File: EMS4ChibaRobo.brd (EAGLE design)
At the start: 51 x 51.5 mm, 31 parts, among them CON1 XT60PB-F, CON2 XT60PB-M, CON3 XT60PB-M, Q2 BUZ11BH, U1 V23134J1052D642, U10 MC34063AD, U4 TLP184, U9 XC6206

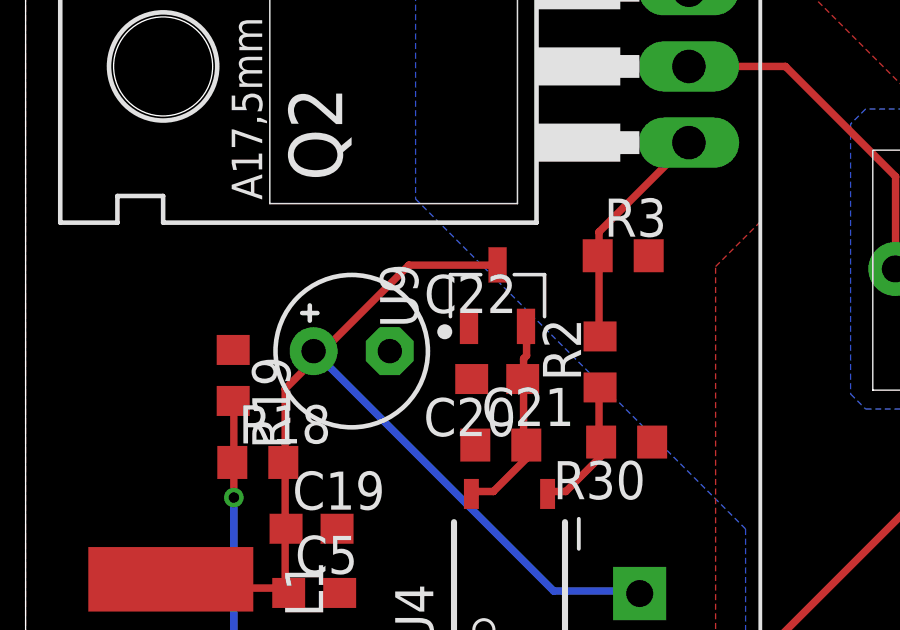
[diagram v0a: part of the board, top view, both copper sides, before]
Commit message: 微調整
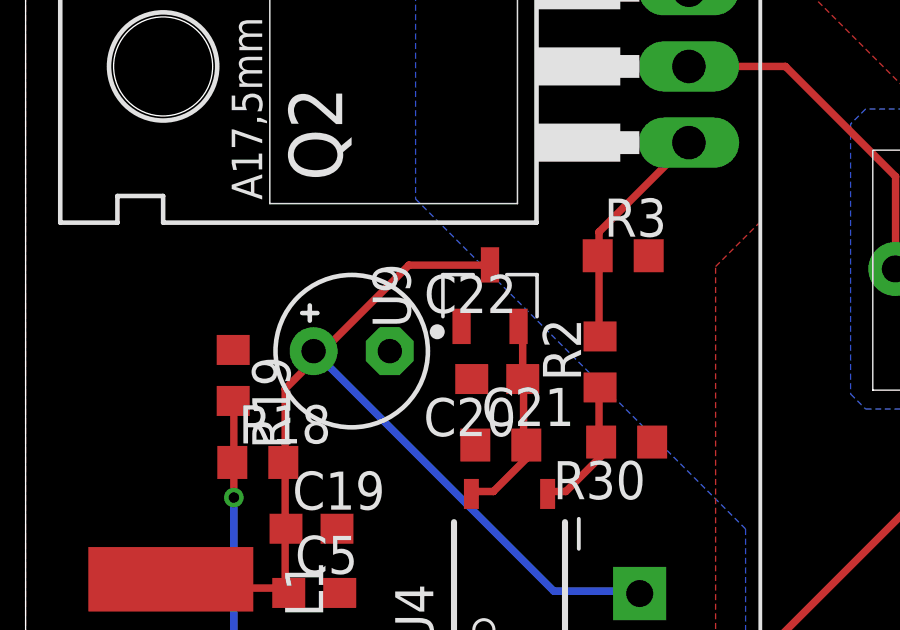
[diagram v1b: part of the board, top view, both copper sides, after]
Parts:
- moved U9 0.25 mm to (15.5, 57.0)
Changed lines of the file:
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@@
 <attribute name="VALUE" x="19.94" y="45.275" size="1.27" layer="27" rot="R90"/>
 </element>
-<element name="U9" library="torex" package="SOT95P240X110-3" package3d_urn="urn:adsk.eagle:package:6993131/1" value="XC6206" x="15.73" y="57.03" smashed="yes" rot="R90">
-<attribute name="NAME" x="13.0864" y="57.03" size="1.27" layer="25" rot="R90" align="bottom-center"/>
-<attribute name="VALUE" x="17.9336" y="57.03" size="1.27" layer="27" rot="R90" align="top-center"/>
+<element name="U9" library="torex" package="SOT95P240X110-3" package3d_urn="urn:adsk.eagle:package:6993131/1" value="XC6206" x="15.48" y="57.03" smashed="yes" rot="R90">
+<attribute name="NAME" x="12.8364" y="57.03" size="1.27" layer="25" rot="R90" align="bottom-center"/>
+<attribute name="VALUE" x="17.6836" y="57.03" size="1.27" layer="27" rot="R90" align="top-center"/>
 </element>
 <element name="C19" library="rcl" library_urn="urn:adsk.eagle:library:334" package="C0603" package3d_urn="urn:adsk.eagle:package:23616/2" value="1u" x="9.53" y="49.26" smashed="yes">
@@
 <contactref element="U9" pad="2"/>
 <contactref element="C20" pad="1"/>
-<wire x1="16.599" y1="54.9276" x2="16.599" y2="54.324" width="0.25" layer="1"/>
-<wire x1="16.6996" y1="55.0282" x2="16.599" y2="54.9276" width="0.25" layer="1"/>
-<wire x1="16.6996" y1="55.9336" x2="16.6996" y2="55.0282" width="0.25" layer="1"/>
-<wire x1="16.599" y1="54.324" x2="16.57" y2="54.25" width="0.25" layer="1"/>
-<wire x1="16.6996" y1="55.9336" x2="16.68" y2="56.0055" width="0.25" layer="1"/>
 <wire x1="15.593" y1="50.5012" x2="14.8888" y2="50.5012" width="0.25" layer="1"/>
 <wire x1="16.6996" y1="51.6078" x2="15.593" y2="50.5012" width="0.25" layer="1"/>
@@
 <wire x1="16.599" y1="54.2234" x2="16.57" y2="54.25" width="0.25" layer="1"/>
 <wire x1="16.599" y1="52.1108" x2="16.69" y2="52.05" width="0.25" layer="1"/>
+<wire x1="16.57" y1="54.25" x2="16.57" y2="55.8655" width="0.25" layer="1"/>
+<wire x1="16.57" y1="55.8655" x2="16.43" y2="56.0055" width="0.25" layer="1"/>
 </signal>
 <signal name="N$30">
@@
 <wire x1="8.551" y1="47.282" x2="8.77" y2="47.12" width="0.25" layer="1"/>
 <wire x1="4.9294" y1="47.4832" x2="4.84" y2="47.575" width="0.25" layer="1"/>
-<wire x1="12.7762" y1="58.0462" x2="15.6936" y2="58.0462" width="0.25" layer="1"/>
+<wire x1="12.7762" y1="58.0462" x2="15.4436" y2="58.0462" width="0.25" layer="1"/>
 <wire x1="9.9594" y1="55.2294" x2="12.7762" y2="58.0462" width="0.25" layer="1"/>
 <wire x1="9.6576" y1="55.2294" x2="9.9594" y2="55.2294" width="0.25" layer="1"/>
-<wire x1="15.6936" y1="58.0462" x2="15.73" y2="58.0545" width="0.25" layer="1"/>
+<wire x1="15.4436" y1="58.0462" x2="15.48" y2="58.0545" width="0.25" layer="1"/>
 <wire x1="9.6576" y1="55.2294" x2="9.6" y2="55.18" width="0.25" layer="1"/>
 <wire x1="17.605" y1="47.1814" x2="20.4218" y2="47.1814" width="0.25" layer="16"/>

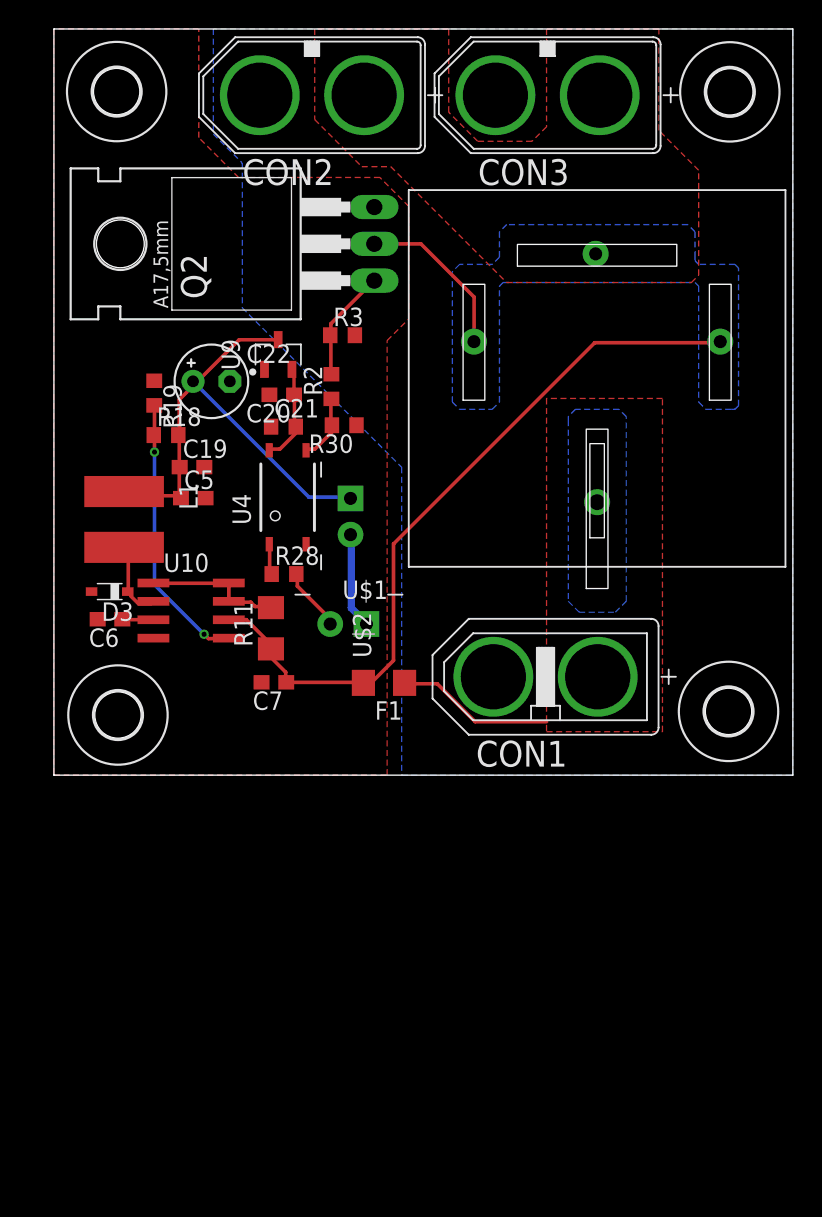
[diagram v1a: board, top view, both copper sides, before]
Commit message: 大幅な設計変更
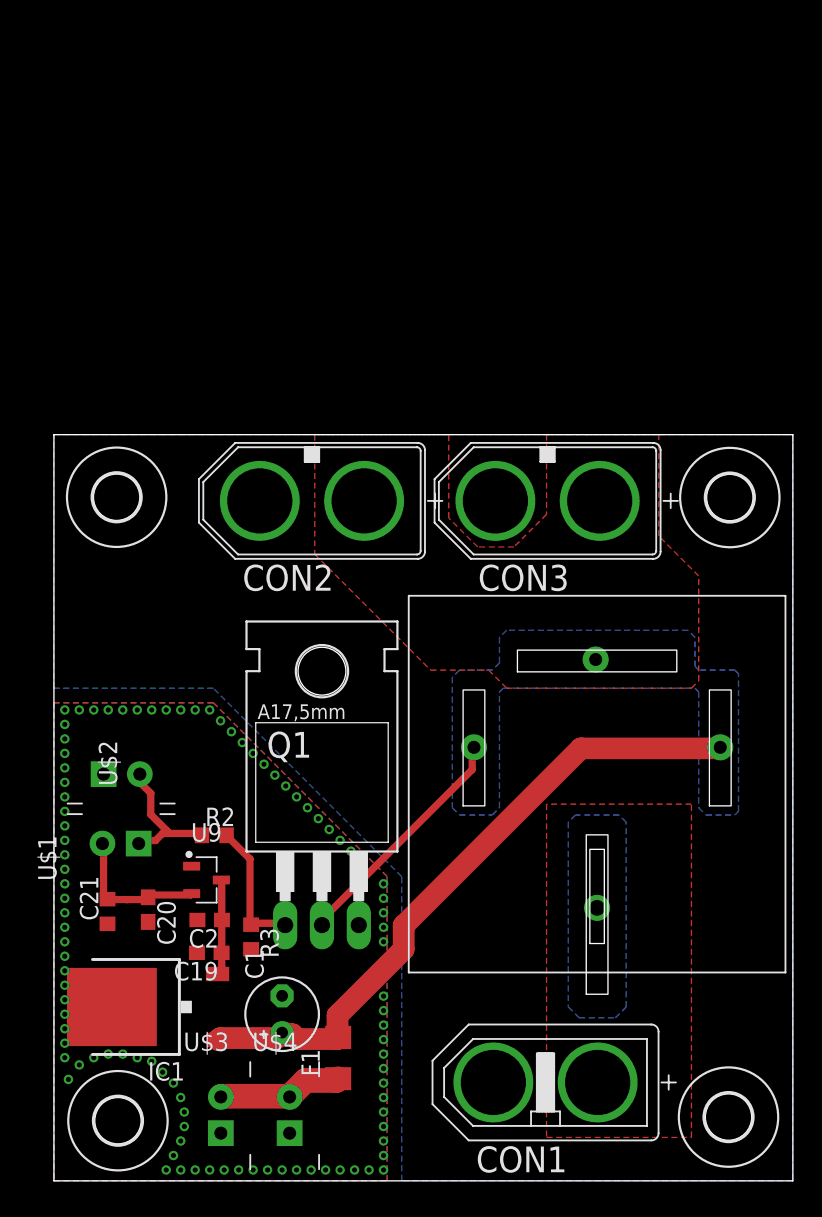
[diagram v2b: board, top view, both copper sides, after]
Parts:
- removed C22: 47u, rcl:E2,5-5
- removed C5, C7: 100n, rcl:C0603
- removed C6: 100p, rcl:C0603
- removed D3: PMEG6010CEJ,115, nexperia:SOD323_ST
- removed L1: L5852, inductors:L5852
- removed Q2: BUZ11BH, transistor-power:TO220BH
- removed R11: 0.68, rcl:R1206
- removed R18: 3.6k, rcl:R0603
- removed R19: 1.2k, rcl:R0603
- removed R28, R30: 1k, rcl:R0603
- removed U10: MC34063AD, mc34063:SOIC8
- removed U4: TLP184, md201x:11-4M1S
- added C1: 22u, rcl:E2,5-5
- added C2: 100n, rcl:C0603
- added IC1: 7805DT, linear:TO252
- added Q1: BUZ11BH, transistor-power:TO220BH
- added U$3, U$4: XH-2-STRAIGHT, con-xh:CON-XH-2-STRAIGHT
- moved R3 42.0 mm to (13.6, 16.8), turned to 270 degrees
- moved C20 36.7 mm to (6.50, 18.7), turned to 270 degrees
- moved U9 36.6 mm to (10.5, 20.8), turned to 0 degrees
- moved C21 35.6 mm to (3.70, 18.6), turned to 90 degrees
- moved C19 33.5 mm to (10.7, 15.7), turned to 180 degrees
- moved R2 32.0 mm to (11.1, 23.9), turned to 0 degrees
- moved CON2 28.0 mm to (17.8, 46.9)
- moved CON3 28.0 mm to (34.1, 46.9)
- moved H1 28.0 mm to (4.33, 47.2)
- moved U1 28.0 mm to (37.5, 27.4)
- moved CON1 28.0 mm to (33.9, 6.79)
- moved H2 28.0 mm to (46.6, 47.2)
- moved H3 28.0 mm to (46.6, 4.40)
- moved H4 28.0 mm to (4.42, 4.15)
- moved U$1 26.6 mm to (4.64, 24.0), turned to 0 degrees
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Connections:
- removed net N$1: R11.2, U10.1, U10.7, U10.8
- removed net N$26: D3.C, L1.P$1, U10.2
- removed net N$27: C6.1, U10.3
- removed net N$28: R18.1, R19.2, U10.5
- removed net N$30: R28.1, U4.1
- removed net SEND_EMS: U$1.P$2, U$2.P$1
- new net LOG_OUT: F1.1, U$3.P$2, U$4.P$2
- net !EMS: now also U$1.P$1; no longer R30.2, U4.3
- net !EMS_ISO: no longer R28.2
- net +12V: now also C1.+, IC1.1; no longer C7.1, R11.1, U10.6
- net +3V3: now also U$1.P$2; no longer U4.4
- net +5V: now also C2.1, IC1.2; no longer C22.+, C5.1, L1.P$2, R18.2, U$1.P$1
- net BATT_POWER: no longer F1.1
- net GNDIO: now also C1.-, C2.2, IC1.3, Q1.S, U$2.P$1, U$3.P$1, U$4.P$1; no longer C22.-, C5.2, C6.2, C7.2, D3.A, Q2.S, R19.1, R30.1, U10.4, U4.2
- net N$6: now also Q1.D; no longer Q2.D
- net N$7: now also Q1.G; no longer Q2.G
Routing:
- net +5V: track 34.0 -> 6.79 mm
- net N$28: track 19.1 -> 0.00 mm, vias 2 -> 0
- net BATT_POWER: track 10.9 -> 0.00 mm
- net N$1: track 9.72 -> 0.00 mm
- net LOG_OUT: track 0.00 -> 8.72 mm
- net SEND_EMS: track 6.62 -> 0.00 mm
- net +12V: track 51.1 -> 45.3 mm
- net N$26: track 5.44 -> 0.00 mm
- net N$6: track 11.5 -> 16.6 mm
- net !EMS_ISO: track 4.43 -> 0.00 mm
- net !EMS: track 4.71 -> 8.89 mm
- net +3V3: track 6.87 -> 10.2 mm
- net N$27: track 2.17 -> 0.00 mm
- net N$30: track 2.12 -> 0.00 mm
- net N$7: track 7.76 -> 9.30 mm
- added copper zone on layer 16, net GNDIO
